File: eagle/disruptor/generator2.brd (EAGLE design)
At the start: 76.2 x 120.7 mm, 29 parts, among them IC1 NE555, IC2 74ALS04N, IC3 IR2110, IC4 7805TV, J1 PIN2F061.100, J2 PIN2F061.100, J3 PIN2F061.100, J4 PIN2F061.100, J5 PIN2F061.100, J6 PIN2F061.100, Q1 STP11NM60, Q2 STP11NM60

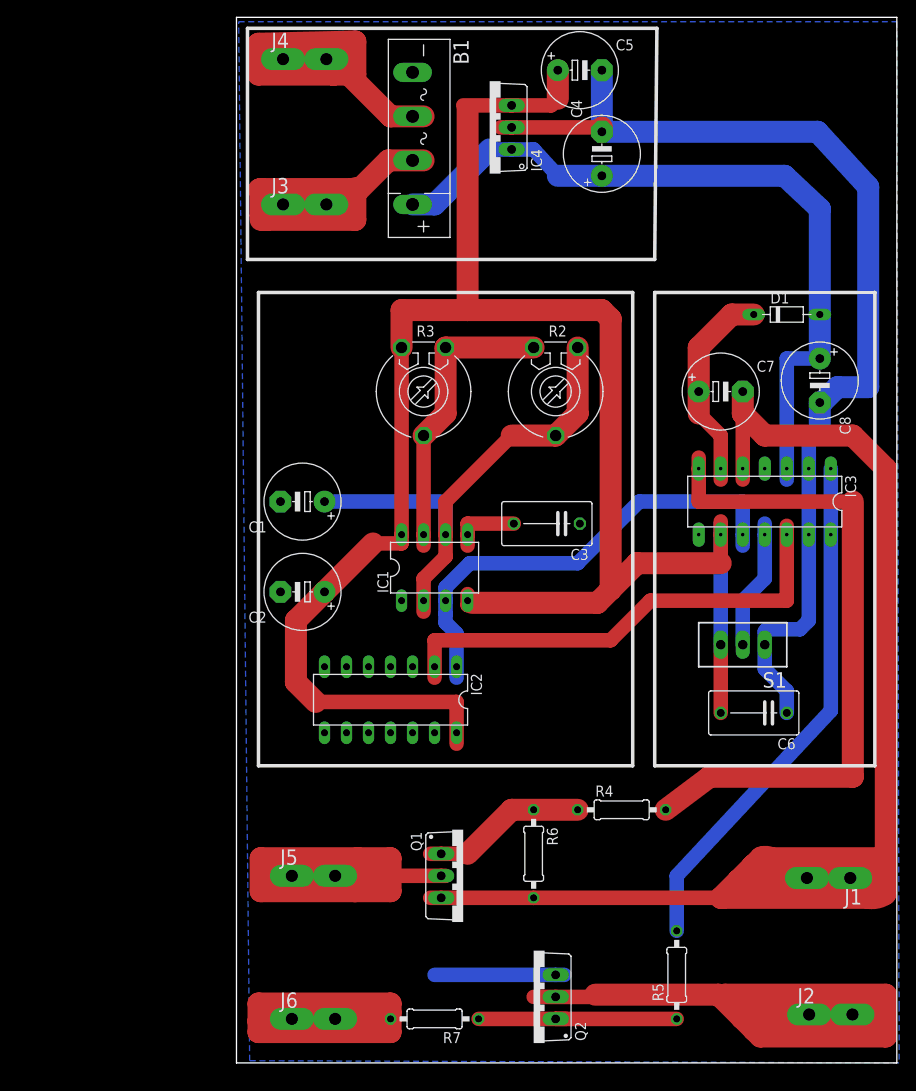
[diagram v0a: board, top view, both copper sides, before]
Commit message: rev2
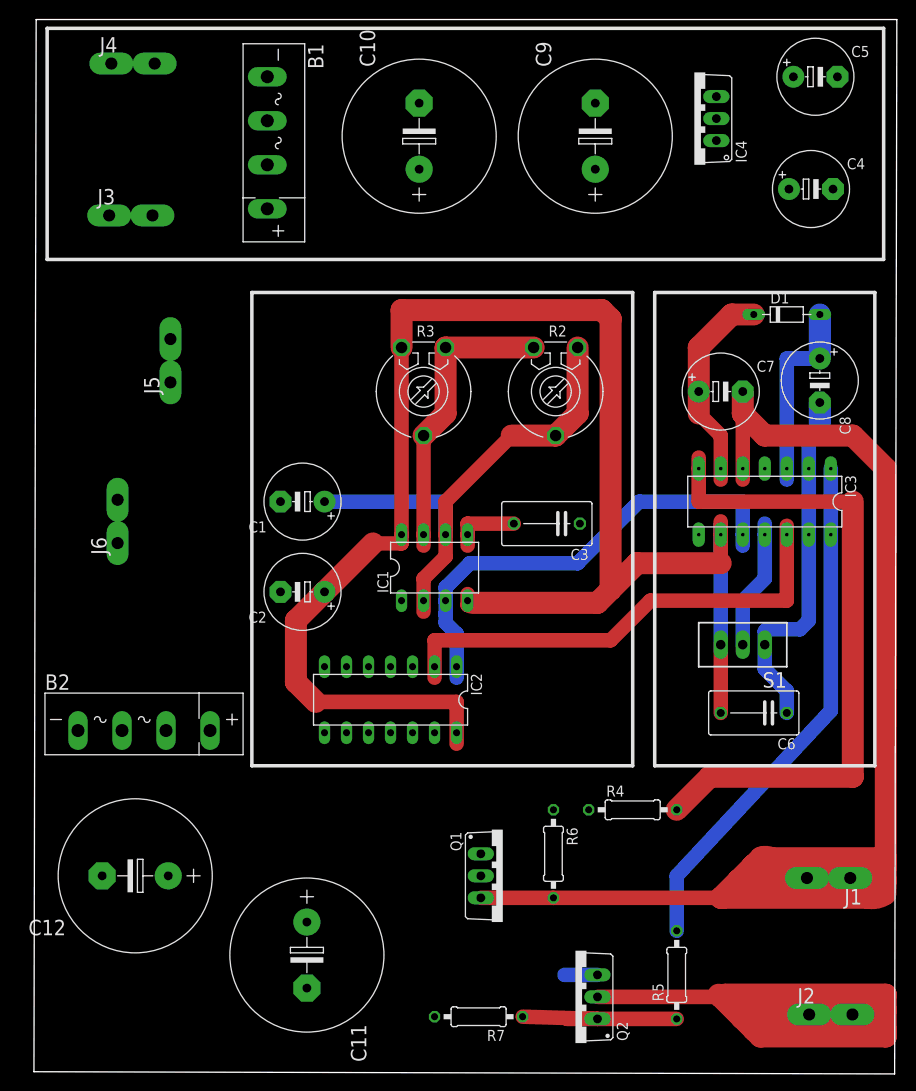
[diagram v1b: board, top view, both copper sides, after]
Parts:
- added B2: RECTIFIER-GBU4, rectifier:GBU4
- added C10, C11, C12, C9: (no value), resistor:E7,5-18
- R4, R5: value (none) -> 100
- R6, R7: value (none) -> 1M
- moved J6 61.7 mm to (-13.7, 62.5), turned to 90 degrees
- moved J5 61.7 mm to (-7.62, 81.0), turned to 90 degrees
- moved C5 27.2 mm to (66.8, 113.8)
- moved C4 24.5 mm to (66.3, 100.8), turned to 0 degrees
- moved IC4 23.6 mm to (52.8, 109.0)
- moved J3 20.1 mm to (-12.2, 97.8)
- moved J4 19.8 mm to (-11.9, 115.3)
- moved B1 16.8 mm to (3.56, 106.2)
- moved R7 5.09 mm to (27.9, 5.33)
- moved Q2 4.83 mm to (39.1, 7.62)
- moved Q1 4.57 mm to (30.7, 21.6)
- moved R6 2.29 mm to (36.6, 24.1)
- moved R4 1.27 mm to (45.7, 29.2)
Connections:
- removed net N$13: J5.A1, J5.A2, Q1.D
- new net N$4: B2.AC1, J5.A1, J5.A2
- new net N$5: B2.AC2, J6.A1, J6.A2
- new net N$6: B2.+, C11.+, C12.+, Q1.D
- net GND: now also B2.-, C10.-, C11.-, C12.-, C9.-; no longer J6.A1, J6.A2
- net VDD: now also C10.+, C9.+
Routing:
- net GND: track 190.0 -> 45.5 mm
- net VDD: track 87.5 -> 22.9 mm
- net N$13: track 62.5 -> 0.00 mm
- net N$9: track 60.0 -> 0.00 mm
- net N$10: track 54.8 -> 0.00 mm
- net VCC: track 228.9 -> 191.3 mm
- net TRANS2: track 114.5 -> 92.9 mm
- net N$12: track 19.1 -> 0.00 mm
- net TRANS1: track 201.4 -> 195.6 mm
- net N$11: track 24.1 -> 21.3 mm
- net HO: track 77.5 -> 76.5 mm
- removed copper zone on layer 16, net GND
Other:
- board size 76.2 x 120.7 mm -> 99.6 x 121.7 mm
